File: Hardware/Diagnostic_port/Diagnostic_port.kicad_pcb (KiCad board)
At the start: 2 copper layers, 60 x 40 mm, 4 parts

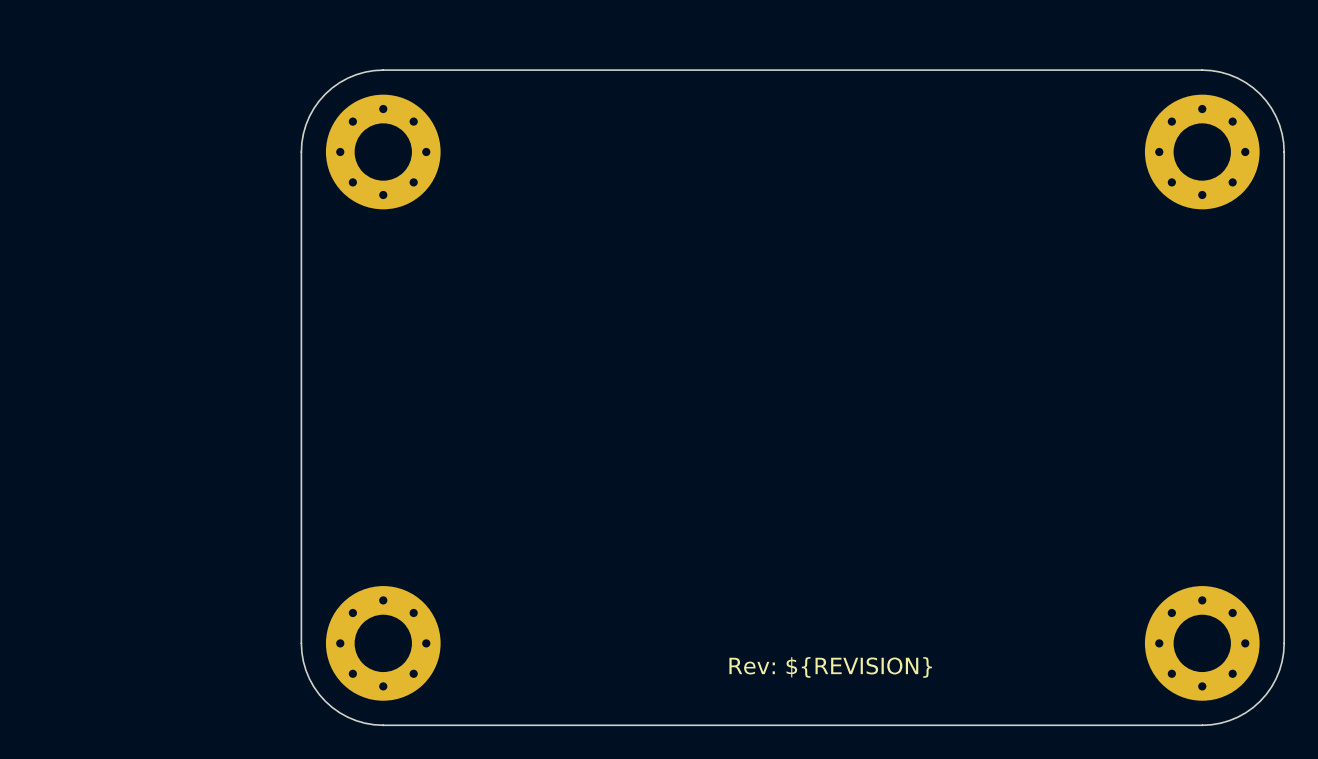
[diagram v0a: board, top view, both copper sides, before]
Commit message: Layout mostly done
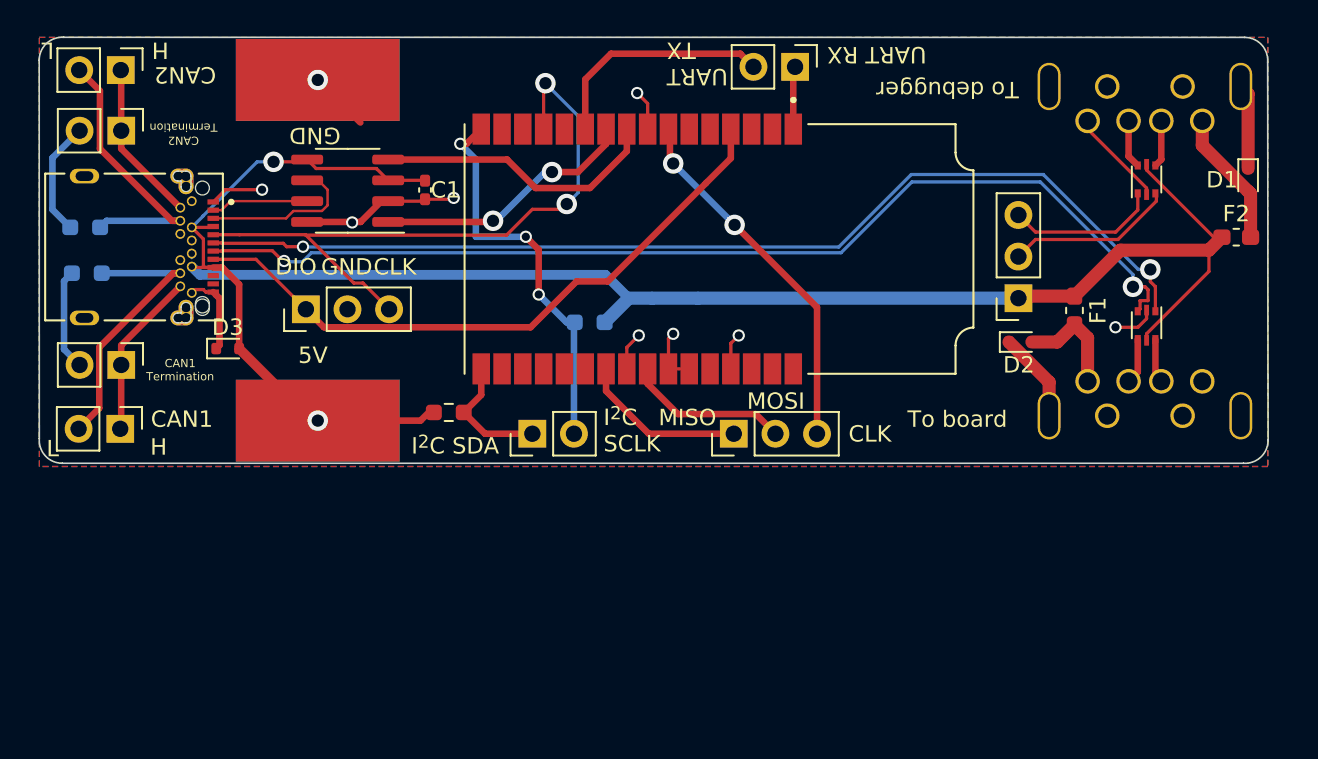
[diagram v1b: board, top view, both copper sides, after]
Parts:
- removed REF** (x4): MountingHole_3.5mm_Pad_Via, MountingHole:MountingHole_3.5mm_Pad_Via
- added ?: , , B.Cu at (117.0, 76.6)
- added C1: 100n, Capacitor_SMD:C_0402_1005Metric_Pad0.74x0.62mm_HandSolder, F.Cu at (123.5, 83.3)
- added D1: 5V, Diode_SMD:D_SOD-523, F.Cu at (173.8, 82.7)
- added D2: 5V, Diode_SMD:D_SOD-523, F.Cu at (159.9, 92.6)
- added D3: 5V, Diode_SMD:D_SOD-523, F.Cu at (111.5, 93.0)
- added F1: 200mA, Fuse:Fuse_0603_1608Metric_Pad1.05x0.95mm_HandSolder, F.Cu at (163.2, 90.7)
- added F2: 200mA, Fuse:Fuse_0603_1608Metric_Pad1.05x0.95mm_HandSolder, F.Cu at (173.1, 86.2)
- added G***: LOGO, Logos:PUTM_LOGO_30mm, B.Cu at (144.3, 83.5)
- added J1: USB_C_Receptacle, frontbox:CUI_UJ31-CH-31-SMT-TR, F.Cu at (110.6, 86.8)
- added J10: Conn_01x02, Connector_PinSocket_2.54mm:PinSocket_1x03_P2.54mm_Vertical, F.Cu at (159.8, 89.9)
- added J11: Conn_01x01_Pin, Connector_Wire:SolderWirePad_1x01_SMD_5x10mm, F.Cu at (117.0, 97.4)
- added J11: Conn_01x01_Pin, Connector_Wire:SolderWirePad_1x01_SMD_5x10mm, B.Cu at (117.0, 97.4)
- added J12: Conn_01x01_Pin, Connector_Wire:SolderWirePad_1x01_SMD_5x10mm, F.Cu at (117.0, 76.6)
- added J2: Conn_01x02, Connector_PinHeader_2.54mm:PinHeader_1x02_P2.54mm_Vertical, F.Cu at (130.1, 98.2)
- added J3: Conn_01x02, Connector_PinHeader_2.54mm:PinHeader_1x02_P2.54mm_Vertical, F.Cu at (146.1, 75.8)
- added J4: Conn_01x04, Connector_PinHeader_2.54mm:PinHeader_1x03_P2.54mm_Vertical, F.Cu at (142.4, 98.2)
- added J5: Conn_01x02, Connector_PinHeader_2.54mm:PinHeader_1x02_P2.54mm_Vertical, F.Cu at (104.9, 97.9)
- added J6: Conn_01x02, Connector_PinHeader_2.54mm:PinHeader_1x02_P2.54mm_Vertical, F.Cu at (105.0, 76.0)
- added J7: Conn_01x03, Connector_PinHeader_2.54mm:PinHeader_1x03_P2.54mm_Vertical, F.Cu at (116.3, 90.6)
- added J8: USB_A, Diag_port:UP2-AH-TH, F.Cu at (167.5, 95.0)
- added J9: USB_A, Diag_port:UP2-AH-TH, F.Cu at (167.5, 79.1)
- added JP1: Jumper_2_Open, Connector_PinHeader_2.54mm:PinHeader_1x02_P2.54mm_Vertical, F.Cu at (105.0, 94.0)
- added JP2: Jumper_2_Open, Connector_PinHeader_2.54mm:PinHeader_1x02_P2.54mm_Vertical, F.Cu at (105.0, 79.7)
- added R1: 120R, Resistor_SMD:R_0603_1608Metric_Pad0.98x0.95mm_HandSolder, B.Cu at (102.9, 88.4)
- added R2: 120R, Resistor_SMD:R_0603_1608Metric_Pad0.98x0.95mm_HandSolder, B.Cu at (102.8, 85.6)
- added R3: 680R, Resistor_SMD:R_0603_1608Metric_Pad0.98x0.95mm_HandSolder, B.Cu at (133.6, 91.4)
- added R4: 680R, Resistor_SMD:R_0603_1608Metric_Pad0.98x0.95mm_HandSolder, F.Cu at (125.0, 96.9)
- added U1: ~, Diag_port:MODULE_STLINK-V3MODS, F.Cu at (155.9, 86.9)
- added U2: ATA6561-GAQW-N, Package_SO:SOIC-8_3.9x4.9mm_P1.27mm, F.Cu at (118.8, 83.4)
- added U3: USBLC6-2P6, Package_TO_SOT_SMD:SOT-666, F.Cu at (167.6, 91.6)
- added U4: USBLC6-2P6, Package_TO_SOT_SMD:SOT-666, F.Cu at (167.6, 82.7)
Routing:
- net +5V: track 0.00 -> 123.2 mm, vias 0 -> 2
- net /USB_D+: track 0.00 -> 64.5 mm, vias 0 -> 2
- net /USB_D-: track 0.00 -> 64.4 mm, vias 0 -> 2
- net GND: track 0.00 -> 52.0 mm, vias 0 -> 9
- net /SWCLK: track 0.00 -> 40.7 mm, vias 0 -> 2
- net /SWDIO: track 0.00 -> 39.4 mm
- net /CAN1_L: track 0.00 -> 26.9 mm
- net /EXT_I2C_SCLK: track 0.00 -> 24.3 mm, vias 0 -> 3
- net /EXT_SPI_CLK: track 0.00 -> 22.4 mm, vias 0 -> 2
- net /TARGET_CAN_RX: track 0.00 -> 17.6 mm
- net /CAN2_L: track 0.00 -> 17.1 mm
- net /TARGET_CAN_TX: track 0.00 -> 16.2 mm, vias 0 -> 2
- net /CAN1_H: track 0.00 -> 16.2 mm
- net /EXT_UART_TX: track 0.00 -> 14.3 mm
- net /DEBUGGER_USB_D-: track 0.00 -> 10.3 mm
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- added copper zone on B.Cu, net GND
- added copper zone on F.Cu, net GND
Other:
- board size 60 x 40 mm -> 75 x 26 mm
- board text added: "5 V"
- board text added: "5V"
- board text added: "CAN1"
- board text added: "CAN1 Termination"
- board text added: "CAN2"
- board text added: "CAN2 Termination"
- board text added: "CLK"
- board text added: "DIO"
- board text added: "GND"
- board text added: "H"
- board text added: "I^{2}C SCLK"
- board text added: "I^{2}C SDA"
- board text added: "L"
- board text added: "MISO"
- board text added: "MOSI"
- board text added: "PC side fused at 300 mA, TVS and ESD protected"
- board text added: "To board"
- board text added: "To debugger"
- board text added: "UART RX"
- board text added: "UART TX"
- board text removed: "Rev: ${REVISION}"
